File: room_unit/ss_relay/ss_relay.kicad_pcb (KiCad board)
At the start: 2 copper layers, 26 parts, among them J1 DC Load, J2 AC220, P1 CONN_01X02, Q1 IRF730, U1 PC817

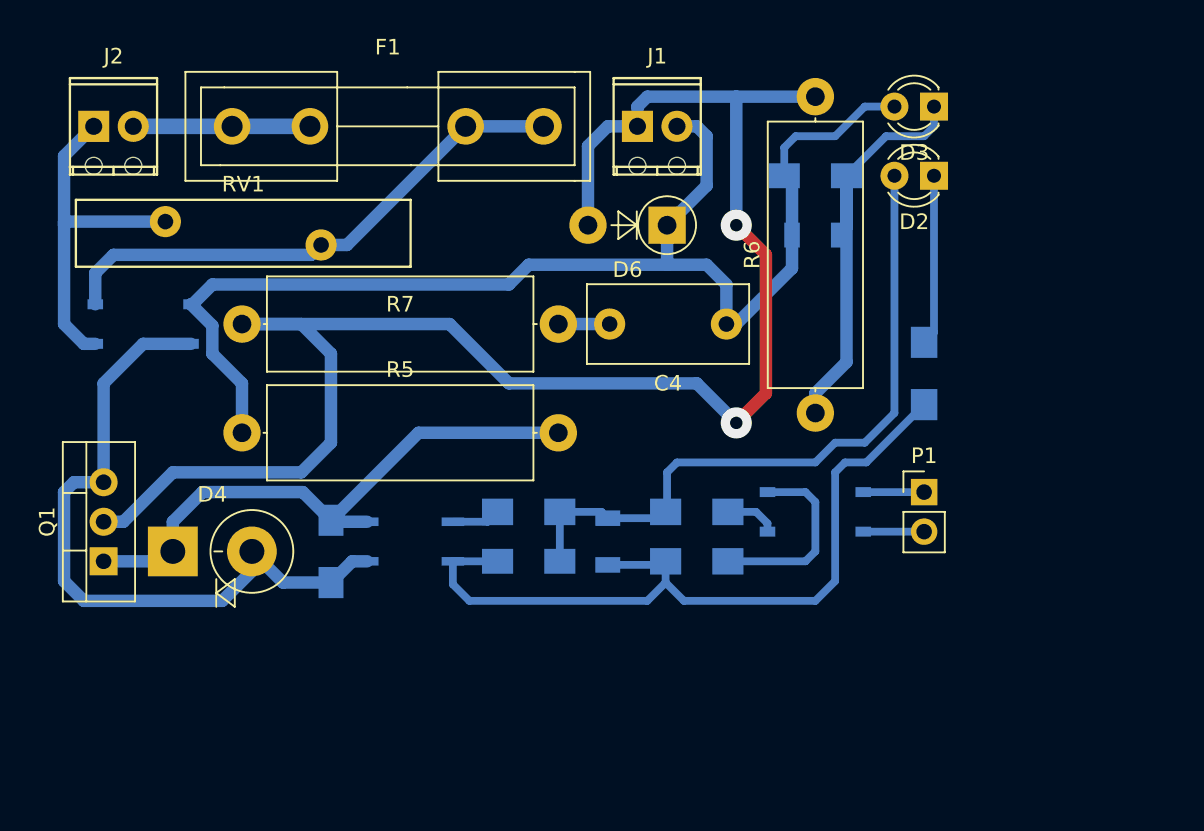
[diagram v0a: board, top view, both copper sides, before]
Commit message: up
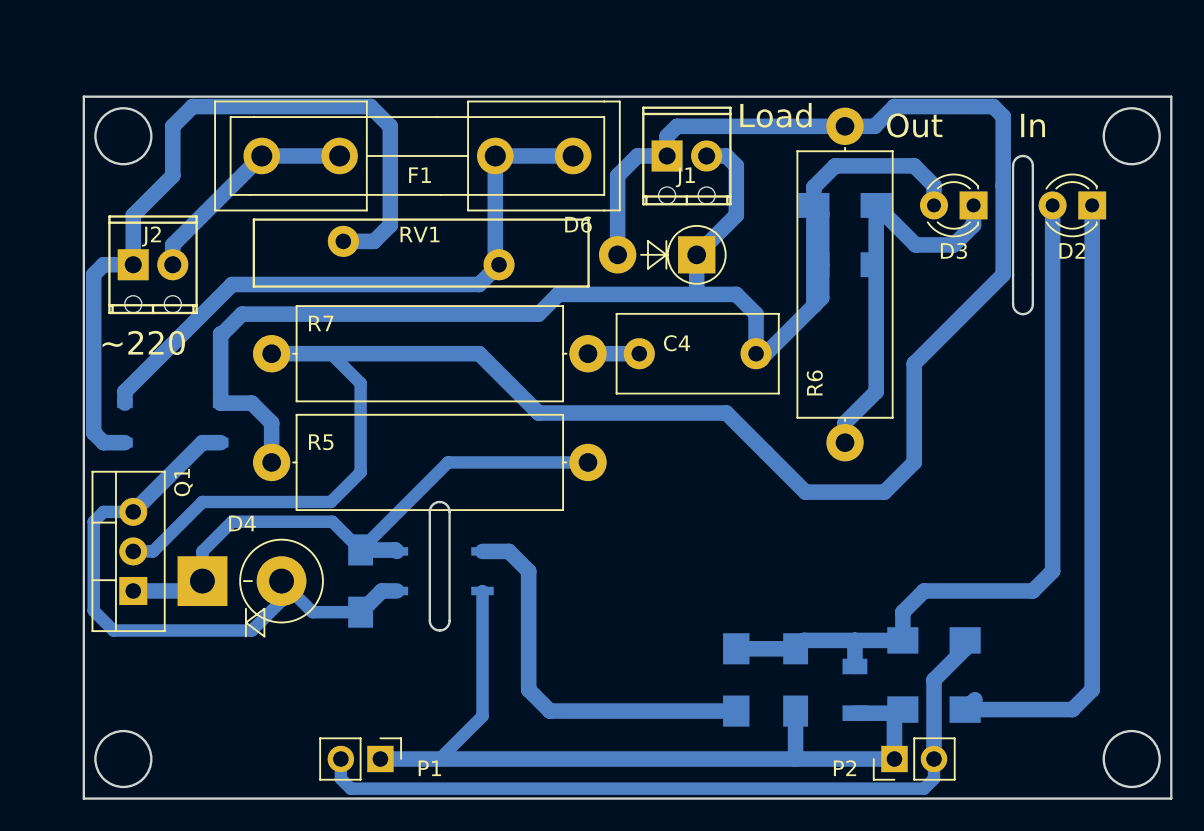
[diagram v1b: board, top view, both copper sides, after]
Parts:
- removed D1: MB6S, Diodes_SMD:Diode_Bridge_TO-269AA
- removed R2: 560, Resistors_SMD:R_1206_HandSoldering
- added P2: DI_B, Pin_Headers:Pin_Header_Straight_1x02_Pitch2.54mm, F.Cu at (148.6, 120.7)
- P1: value CONN_01X02 -> DI_A
- R1: value 560 -> 1k
- moved P1 38.9 mm to (115.6, 120.7), turned to 270 degrees
- moved R3 21.6 mm to (151.1, 117.5), turned to 180 degrees
- moved C1 18.8 mm to (142.2, 115.6), turned to 270 degrees
- moved D8 18.5 mm to (146.1, 116.2)
- moved R1 17.3 mm to (151.1, 113.0)
- moved R4 17.2 mm to (138.4, 115.6), turned to 90 degrees
- moved RV1 11.5 mm to (123.2, 88.9)
- moved D2 10.3 mm to (161.3, 85.1)
- moved J2 9.25 mm to (99.7, 88.9)
- moved D3 6.84 mm to (153.7, 85.1)
- moved D7 6.63 mm to (102.2, 99.1)
- moved C2 2.69 mm to (114.3, 109.2)
- moved C3 2.69 mm to (145.4, 85.1)
- moved C4 2.69 mm to (139.7, 94.6)
- moved D4 2.69 mm to (104.1, 109.2)
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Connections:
- P1 pad 1: Net-(D1-Pad3) -> Net-(C1-Pad2)
- P1 pad 2: Net-(D1-Pad4) -> Net-(P1-Pad2)
- R1 pad 2: Net-(D1-Pad1) -> Net-(P1-Pad2)
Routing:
- net Net-(D6-Pad2): track 107.6 -> 168.4 mm, vias 2 -> 0
- net Net-(C3-Pad1): track 81.4 -> 141.1 mm
- net Net-(P1-Pad2): track 0.00 -> 49.6 mm
- net Net-(C1-Pad2): track 50.5 -> 88.3 mm
- net Net-(D2-Pad1): track 11.0 -> 40.7 mm
- net Net-(D7-Pad3): track 22.8 -> 50.0 mm
- net Net-(R4-Pad1): track 3.13 -> 25.0 mm
- net Net-(C3-Pad2): track 28.3 -> 44.0 mm
- net Net-(D1-Pad2): track 12.4 -> 0.00 mm
- net Net-(D7-Pad4): track 34.7 -> 40.2 mm
- net Net-(C1-Pad1): track 44.3 -> 48.6 mm
- net Net-(D1-Pad4): track 3.91 -> 0.00 mm
- net Net-(D1-Pad3): track 3.91 -> 0.00 mm
- net Net-(C2-Pad2): track 45.0 -> 41.4 mm
- net Net-(D1-Pad1): track 3.38 -> 0.00 mm
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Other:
- board outline added: 69.9 x 45.1 mm
- board text added: "In"
- board text added: "Load"
- board text added: "Out"
- board text added: "~~220"
